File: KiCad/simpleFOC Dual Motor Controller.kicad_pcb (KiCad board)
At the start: 4 copper layers, 50 x 50 mm, 55 parts, among them CN101 MR60-F, CN201 MR60-F, CN601 MR60-F, Q301 AGM6014AP, Q303 AGM6014AP, Q401 AGM6014AP, Q403 AGM6014AP, Q501 AGM6014AP, Q503 AGM6014AP, Q701 AGM6014AP, Q703 AGM6014AP, Q801 AGM6014AP, Q803 AGM6014AP, Q901 AGM6014AP, Q903 AGM6014AP, U101 STM32F103C8Tx, U201 DRV8323HRTAT, U601 DRV8323HRTAT

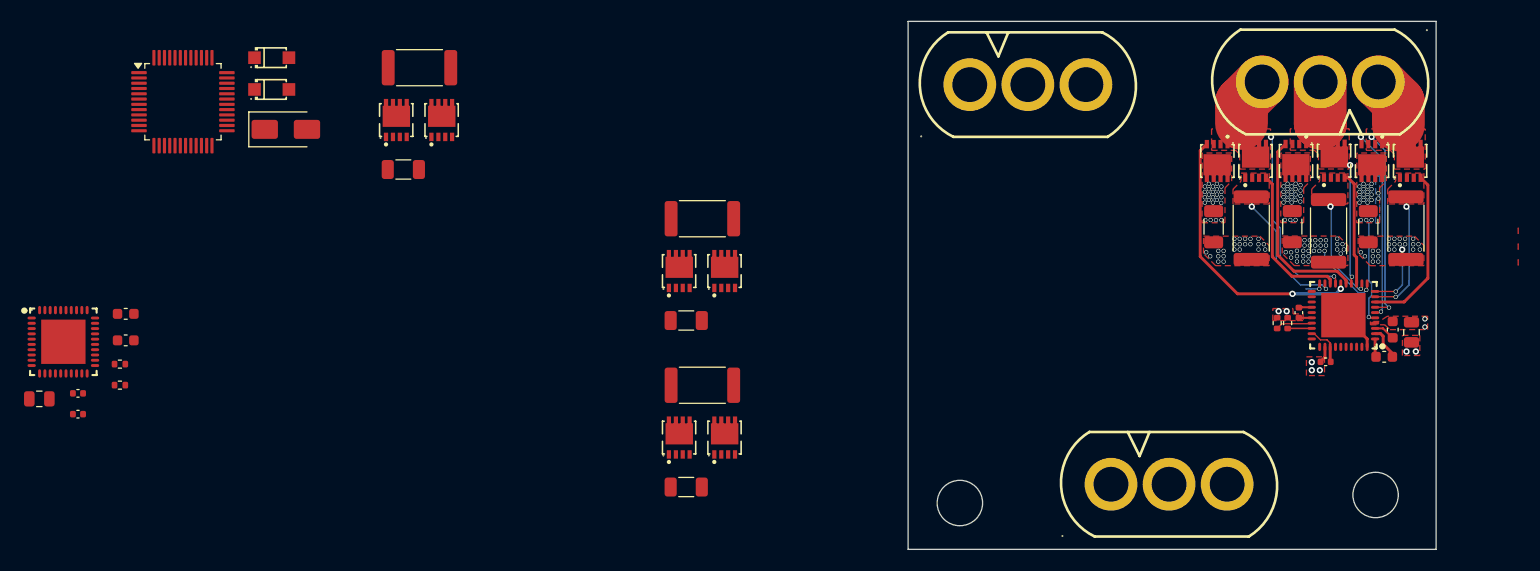
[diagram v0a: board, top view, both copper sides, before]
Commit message: start adding control pins
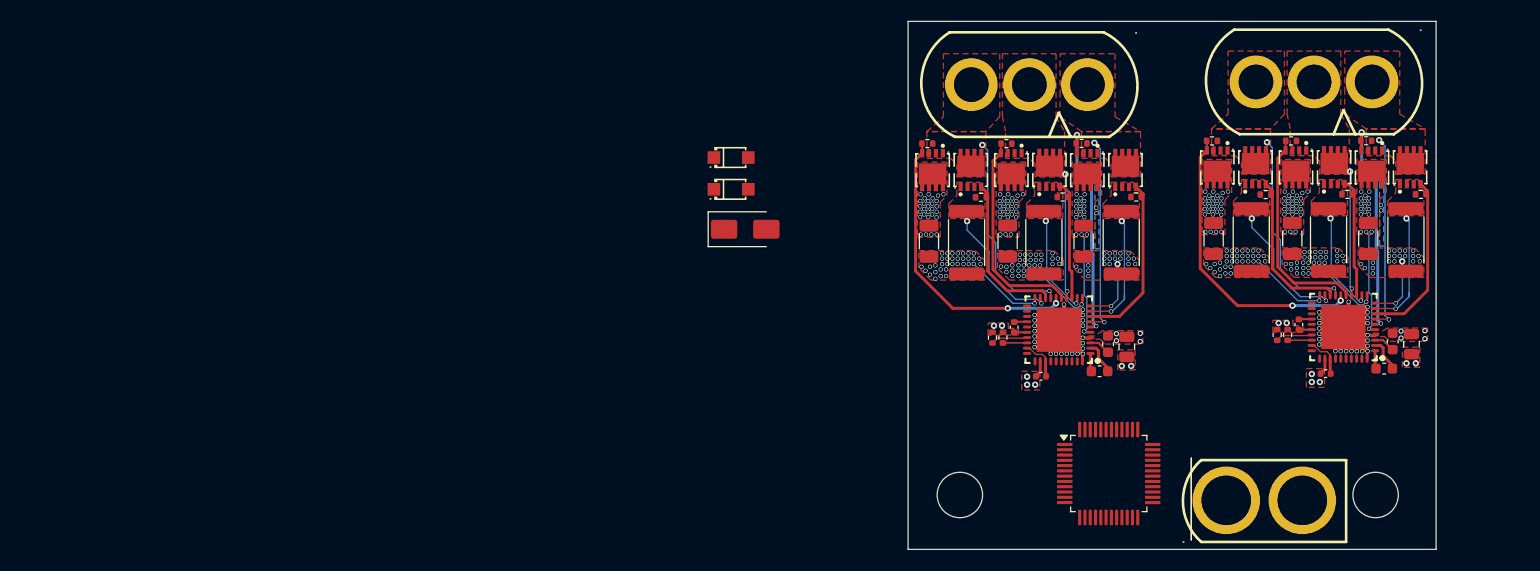
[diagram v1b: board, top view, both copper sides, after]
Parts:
- removed CN101: MR60-F, easyeda2kicad:CONN-TH_3P-P5.50_MR60-F
- added R301: 47k, Resistor_SMD:R_0402_1005Metric, F.Cu at (148.6, 41.4)
- added R302: 47k, Resistor_SMD:R_0402_1005Metric, F.Cu at (143.4, 36.3)
- added R401: 47k, Resistor_SMD:R_0402_1005Metric, F.Cu at (141.6, 41.4)
- added R402: 47k, Resistor_SMD:R_0402_1005Metric, F.Cu at (136.3, 36.3)
- added R501: 47k, Resistor_SMD:R_0402_1005Metric, F.Cu at (133.9, 41.4)
- added R502: 47k, Resistor_SMD:R_0402_1005Metric, F.Cu at (128.8, 36.3)
- added R701: 47k, Resistor_SMD:R_0402_1005Metric, F.Cu at (114.6, 41.6)
- added R702: 47k, Resistor_SMD:R_0402_1005Metric, F.Cu at (109.3, 36.6)
- added R801: 47k, Resistor_SMD:R_0402_1005Metric, F.Cu at (106.9, 41.7)
- added R802: 47k, Resistor_SMD:R_0402_1005Metric, F.Cu at (101.8, 36.6)
- added R901: 47k, Resistor_SMD:R_0402_1005Metric, F.Cu at (121.6, 41.6)
- added R902: 47k, Resistor_SMD:R_0402_1005Metric, F.Cu at (116.4, 36.6)
- added U102: XT60H-M, easyeda2kicad:CONN-TH_XT60H-M, F.Cu at (133.7, 70.4)
- NT601, NT602, NT603: moved to B.Cu
- moved C601 103.1 mm to (120.7, 55.8), turned to -90 degrees
- moved U101 94.5 mm to (119.0, 67.8)
- moved U601 94.3 mm to (114.3, 54.2), turned to 180 degrees
- moved C602 93.1 mm to (118.9, 55.6), turned to -90 degrees
- moved C603 92.3 mm to (118.1, 58.1)
- moved C604 91.2 mm to (112.6, 58.6), turned to 180 degrees
- moved C605 89.0 mm to (110.0, 54.0), turned to -90 degrees
- moved R602 83.7 mm to (109.0, 54.9), turned to 90 degrees
- moved R601 82.7 mm to (108.0, 54.9), turned to 90 degrees
- moved C701 64.8 mm to (116.6, 45.8), turned to -90 degrees
- moved Rsns701 61.4 mm to (112.9, 45.9), turned to -90 degrees
- moved Q701 58.4 mm to (109.8, 39.1), turned to 180 degrees
- moved Q703 57.8 mm to (113.4, 39.1)
- moved NT603 47.0 mm to (111.0, 51.7), turned to -90 degrees
- moved Q901 46.2 mm to (117.0, 39.1), turned to 180 degrees
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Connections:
- C604 pad 2: GND -> /Motor Driver 1/Motor_VIN
- C605 pad 2: GND -> /Motor Driver 1/Motor_VIN
- NT601 pad 2: GND -> /Motor Driver 1/Motor_VIN
- NT602 pad 2: GND -> /Motor Driver 1/Motor_VIN
- NT603 pad 2: GND -> /Motor Driver 1/Motor_VIN
- Rsns401 pad 2: GND -> /Motor Driver 1/Motor_VIN
- Rsns701 pad 2: GND -> /Motor Driver 1/Motor_VIN
- Rsns901 pad 2: GND -> /Motor Driver 1/Motor_VIN
- U201 pad 21: unconnected-(U201-SOC-Pad21) -> /Motor Driver 1/SOC
- U201 pad 22: unconnected-(U201-SOB-Pad22) -> /Motor Driver 1/SOB
- U201 pad 23: unconnected-(U201-SOA-Pad23) -> /Motor Driver 1/SOA
- U201 pad 25: unconnected-(U201-nFAULT-Pad25) -> /Motor Driver 1/FAULT
- U201 pad 30: unconnected-(U201-ENABLE-Pad30) -> /Motor Driver 1/EN
- U201 pad 31: unconnected-(U201-CAL-Pad31) -> /Motor Driver 1/CAL
- U201 pad 34: unconnected-(U201-INHA-Pad34) -> /Motor Driver 1/INHA
- U201 pad 35: unconnected-(U201-INLA-Pad35) -> /Motor Driver 1/INLA
- U201 pad 36: unconnected-(U201-INHB-Pad36) -> /Motor Driver 1/INHB
- U201 pad 37: unconnected-(U201-INLB-Pad37) -> /Motor Driver 1/INLB
- U201 pad 38: unconnected-(U201-INHC-Pad38) -> /Motor Driver 1/INHC
- U201 pad 39: unconnected-(U201-INLC-Pad39) -> /Motor Driver 1/INLC
- U201 pad 40: GND -> /Motor Driver 1/Motor_VIN
- U201 pad 41: GND -> /Motor Driver 1/Motor_VIN
- U601 pad 21: unconnected-(U601-SOC-Pad21) -> /Motor Driver 2/SOC
- U601 pad 22: unconnected-(U601-SOB-Pad22) -> /Motor Driver 2/SOB
- U601 pad 23: unconnected-(U601-SOA-Pad23) -> /Motor Driver 2/SOA
- U601 pad 25: unconnected-(U601-nFAULT-Pad25) -> /Motor Driver 2/FAULT
- U601 pad 26: GND -> /Motor Driver 1/Motor_VIN
- U601 pad 30: unconnected-(U601-ENABLE-Pad30) -> /Motor Driver 2/EN
- U601 pad 31: unconnected-(U601-CAL-Pad31) -> /Motor Driver 2/CAL
- U601 pad 32: GND -> /Motor Driver 1/Motor_VIN
- U601 pad 34: unconnected-(U601-INHA-Pad34) -> /Motor Driver 2/INHA
- U601 pad 35: unconnected-(U601-INLA-Pad35) -> /Motor Driver 2/INLA
- U601 pad 36: unconnected-(U601-INHB-Pad36) -> /Motor Driver 2/INHB
- U601 pad 37: unconnected-(U601-INLB-Pad37) -> /Motor Driver 2/INLB
- U601 pad 38: unconnected-(U601-INHC-Pad38) -> /Motor Driver 2/INHC
- U601 pad 39: unconnected-(U601-INLC-Pad39) -> /Motor Driver 2/INLC
- U601 pad 40: GND -> /Motor Driver 1/Motor_VIN
- U601 pad 41: GND -> /Motor Driver 1/Motor_VIN
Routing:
- net /Motor Driver 1/Motor_VIN: track 14.7 -> 168.9 mm, vias 70 -> 193
- net /Motor Driver 2/Pole 3/GH: track 0.00 -> 27.4 mm, vias 0 -> 2
- net /Motor Driver 2/Pole 1/GH: track 0.00 -> 21.1 mm, vias 0 -> 2
- net /Motor Driver 2/Pole 2/GH: track 0.00 -> 20.0 mm
- net /Motor Driver 2/Pole 3/PoleOut: track 0.00 -> 19.1 mm, vias 0 -> 2
- net /Motor Driver 2/Pole 1/PoleOut: track 0.00 -> 18.7 mm, vias 0 -> 2
- net /Motor Driver 2/Pole 1/GL: track 0.00 -> 16.2 mm
- net /Motor Driver 2/Pole 3/GL: track 0.00 -> 15.0 mm
- net /Motor Driver 2/Pole 2/PoleOut: track 0.00 -> 13.6 mm, vias 0 -> 2
- net /Motor Driver 2/Pole 3/SP: track 0.00 -> 13.4 mm, vias 0 -> 2
- net /Motor Driver 2/Pole 1/SP: track 0.00 -> 12.6 mm, vias 0 -> 2
- net /Motor Driver 2/Pole 2/GL: track 0.00 -> 11.2 mm
- net /Motor Driver 2/Pole 2/SP: track 0.00 -> 10.6 mm, vias 0 -> 2
- net Net-(U601-SNB): track 0.00 -> 6.16 mm, vias 0 -> 1
- net Net-(U601-SNA): track 0.00 -> 5.06 mm, vias 0 -> 1
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- added copper zone on F.Cu, net /Motor Driver 2/Pole 1/PoleOut
- added copper zone on F.Cu, net /Motor Driver 2/Pole 1/SP
- added copper zone on F.Cu, net /Motor Driver 2/Pole 2/PoleOut
- added copper zone on F.Cu, net /Motor Driver 2/Pole 2/SP
- added copper zone on F.Cu, net /Motor Driver 2/Pole 3/PoleOut
- added copper zone on F.Cu, net /Motor Driver 2/Pole 3/SP
